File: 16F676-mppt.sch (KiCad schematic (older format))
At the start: 49 parts, among them J1 S+, J2 S-, J3 VB+, J4 VB-, Q1 BUK9511-55A127, Q2 BUK9511-55A127, Q3 2N2222A, Q4 2N2222A, Q5 2N2907A, SW1 Write OP-AMP DIFF, U1 LM7805_TO220, U2 LM358N, U3 16F676

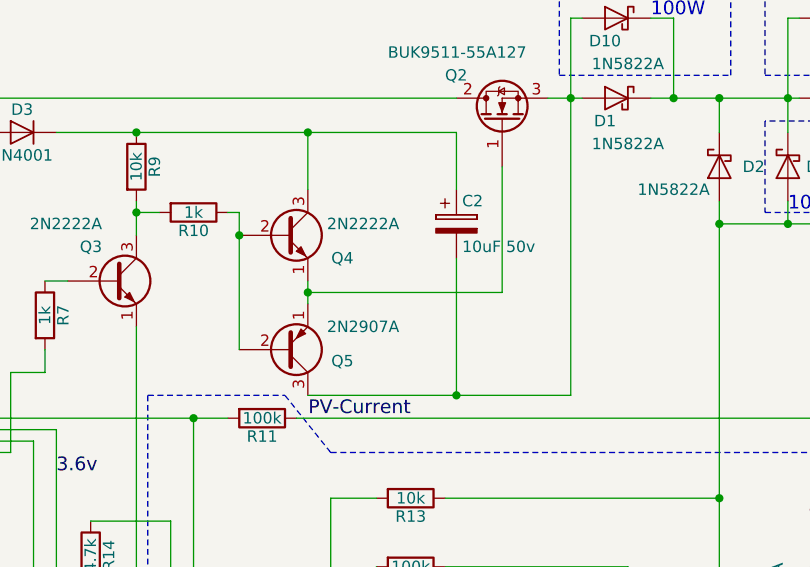
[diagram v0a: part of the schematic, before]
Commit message: Add resistor
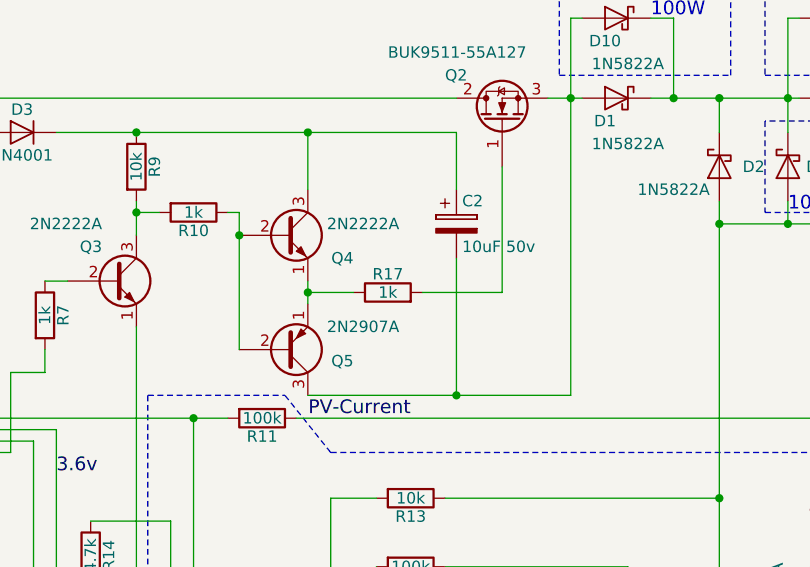
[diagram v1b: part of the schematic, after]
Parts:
- added R17: 1k, Resistors_THT:R_Axial_DIN0309_L9.0mm_D3.2mm_P12.70mm_Horizontal, symbol Device:R
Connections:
- net at Q4.1 (E), Q5.1 (E): now also R17.1; no longer Q2.1 (G)
- new net: Q2.1 (G), R17.2
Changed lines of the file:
@@
 	7900 2200 8000 2200
-Wire Wire Line
-	6850 3000 6850 3050
-Wire Wire Line
-	6850 3050 7700 3050
-Wire Wire Line
-	7700 3050 7700 2500
-Connection ~ 6850 3050
 Wire Wire Line
 	8000 3500 7500 3500
@@
 	8650 2200 8950 2200
 Wire Wire Line
+	8000 2200 8050 2200
+Wire Wire Line
+	7500 3500 6850 3500
+Wire Wire Line
+	6100 5600 5900 5600
+Wire Wire Line
+	6100 2350 6850 2350
+Wire Wire Line
+	6550 2800 6550 3300
+Wire Wire Line
+	6100 2700 6100 2800
+Wire Wire Line
+	1900 2200 2400 2200
+Wire Wire Line
+	2300 5600 1500 5600
+Wire Wire Line
+	1500 2200 1900 2200
+Wire Wire Line
+	1500 3500 1500 3900
+Wire Wire Line
+	4100 5600 2300 5600
+Wire Wire Line
+	2750 4100 3400 4100
+Wire Wire Line
+	2750 3400 3150 3400
+Wire Wire Line
+	3400 4100 4500 4100
+Wire Wire Line
+	3400 3400 3500 3400
+Wire Wire Line
+	6850 2350 7500 2350
+Wire Wire Line
+	7650 5600 7150 5600
+Wire Wire Line
+	7650 4450 8400 4450
+Wire Wire Line
+	8650 2750 8650 3950
+Wire Wire Line
+	9750 2750 10500 2750
+Wire Wire Line
+	9750 2200 10500 2200
+Wire Wire Line
+	1500 5600 1250 5600
+Wire Wire Line
+	6950 5600 6350 5600
+Wire Wire Line
+	6950 4750 6950 5150
+Wire Wire Line
+	8650 3950 8650 5200
+Wire Wire Line
+	5900 5600 5450 5600
+Wire Wire Line
+	6350 5600 6100 5600
+Wire Wire Line
+	6350 3600 6500 3600
+Wire Wire Line
+	5450 5600 4100 5600
+Wire Wire Line
+	5450 4400 5650 4400
+Wire Wire Line
+	5900 4500 5900 4650
+Wire Wire Line
+	5750 4500 5750 6000
+Wire Wire Line
+	8650 5600 7650 5600
+Wire Wire Line
+	9700 4850 9700 5600
+Wire Wire Line
+	8400 4450 8700 4450
+Wire Wire Line
+	9100 3600 9900 3600
+Wire Wire Line
+	2950 2200 7500 2200
+Wire Wire Line
+	2950 2200 2950 2600
+Wire Wire Line
+	3150 5000 3150 6100
+Wire Wire Line
+	3800 4650 3800 5000
+Wire Wire Line
+	2300 4650 2300 5600
+Wire Wire Line
+	2400 2200 2600 2200
+Wire Wire Line
+	8450 2200 8650 2200
+Wire Wire Line
+	8950 2750 9750 2750
+Wire Wire Line
+	8950 2200 8950 2350
+Wire Wire Line
+	8950 2200 9000 2200
+$Comp
+L Device:R R17
+U 1 1 5BF07E56
+P 7200 3050
+F 0 "R17" V 7280 3050 50  0000 C CNN
+F 1 "1k" V 7200 3050 50  0000 C CNN
+F 2 "Resistors_THT:R_Axial_DIN0309_L9.0mm_D3.2mm_P12.70mm_Horizontal" V 7130 3050 30  0001 C CNN
+F 3 "" H 7200 3050 30  0000 C CNN
+	1    7200 3050
+	0    -1   -1   0
+$EndComp
+Wire Wire Line
+	6850 3000 6850 3050
+Wire Wire Line
+	7050 3050 6850 3050
+Wire Wire Line
+	8000 2200 8000 3500
+Connection ~ 6850 3050
+Wire Wire Line
 	6850 3050 6850 3100
 Wire Wire Line
-	8000 2200 8050 2200
-Wire Wire Line
-	8000 2200 8000 3500
-Wire Wire Line
-	7500 3500 6850 3500
-Wire Wire Line
-	6100 5600 5900 5600
-Wire Wire Line
-	6100 2350 6850 2350
-Wire Wire Line
-	6550 2800 6550 3300
-Wire Wire Line
-	6100 2700 6100 2800
-Wire Wire Line
-	1900 2200 2400 2200
-Wire Wire Line
-	2300 5600 1500 5600
-Wire Wire Line
-	1500 2200 1900 2200
-Wire Wire Line
-	1500 3500 1500 3900
-Wire Wire Line
-	4100 5600 2300 5600
-Wire Wire Line
-	2750 4100 3400 4100
-Wire Wire Line
-	2750 3400 3150 3400
-Wire Wire Line
-	3400 4100 4500 4100
-Wire Wire Line
-	3400 3400 3500 3400
-Wire Wire Line
-	6850 2350 7500 2350
-Wire Wire Line
-	7650 5600 7150 5600
-Wire Wire Line
-	7650 4450 8400 4450
-Wire Wire Line
-	8650 2750 8650 3950
-Wire Wire Line
-	9750 2750 10500 2750
-Wire Wire Line
-	9750 2200 10500 2200
-Wire Wire Line
-	1500 5600 1250 5600
-Wire Wire Line
-	6950 5600 6350 5600
-Wire Wire Line
-	6950 4750 6950 5150
-Wire Wire Line
-	8650 3950 8650 5200
-Wire Wire Line
-	5900 5600 5450 5600
-Wire Wire Line
-	6350 5600 6100 5600
-Wire Wire Line
-	6350 3600 6500 3600
-Wire Wire Line
-	5450 5600 4100 5600
-Wire Wire Line
-	5450 4400 5650 4400
-Wire Wire Line
-	5900 4500 5900 4650
-Wire Wire Line
-	5750 4500 5750 6000
-Wire Wire Line
-	8650 5600 7650 5600
-Wire Wire Line
-	9700 4850 9700 5600
-Wire Wire Line
-	8400 4450 8700 4450
-Wire Wire Line
-	9100 3600 9900 3600
-Wire Wire Line
-	2950 2200 7500 2200
-Wire Wire Line
-	2950 2200 2950 2600
-Wire Wire Line
-	3150 5000 3150 6100
-Wire Wire Line
-	3800 4650 3800 5000
-Wire Wire Line
-	2300 4650 2300 5600
-Wire Wire Line
-	2400 2200 2600 2200
-Wire Wire Line
-	8450 2200 8650 2200
-Wire Wire Line
-	8950 2750 9750 2750
-Wire Wire Line
-	8950 2200 8950 2350
-Wire Wire Line
-	8950 2200 9000 2200
+	7350 3050 7700 3050
+Wire Wire Line
+	7700 3050 7700 2500
 $EndSCHEMATC
